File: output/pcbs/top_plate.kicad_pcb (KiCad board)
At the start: 2 copper layers, 162.1 x 157 mm, 0 parts

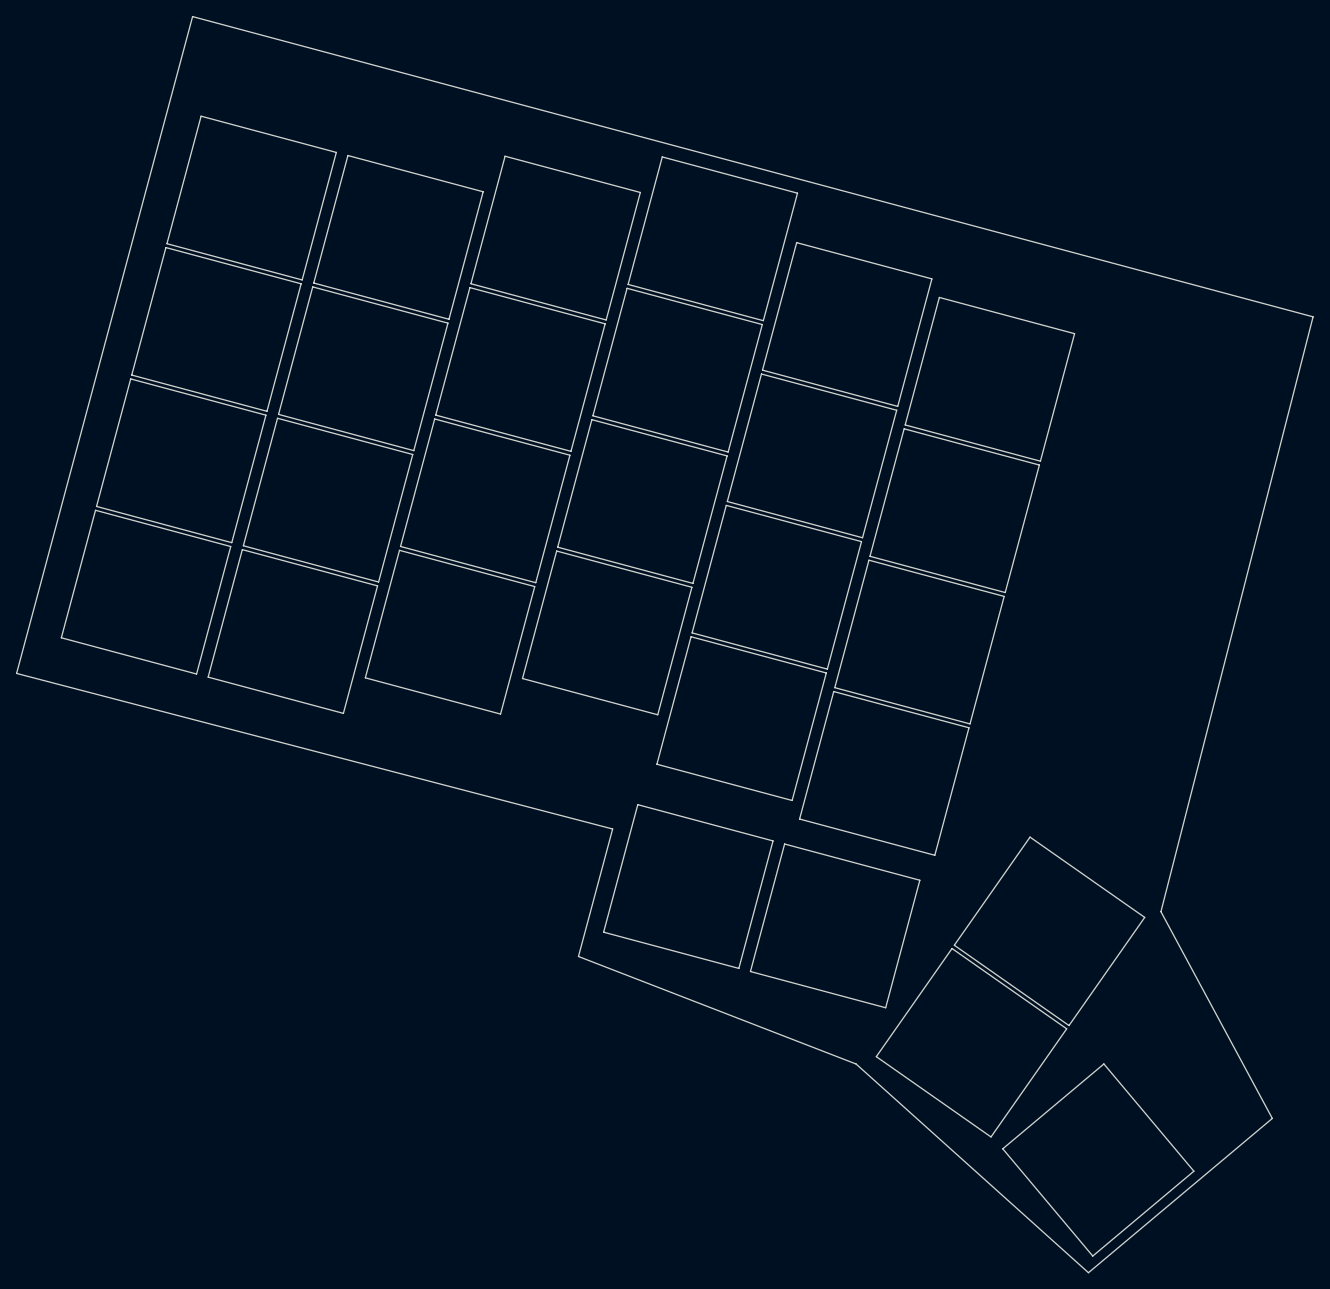
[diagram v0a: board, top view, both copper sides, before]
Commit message: holes
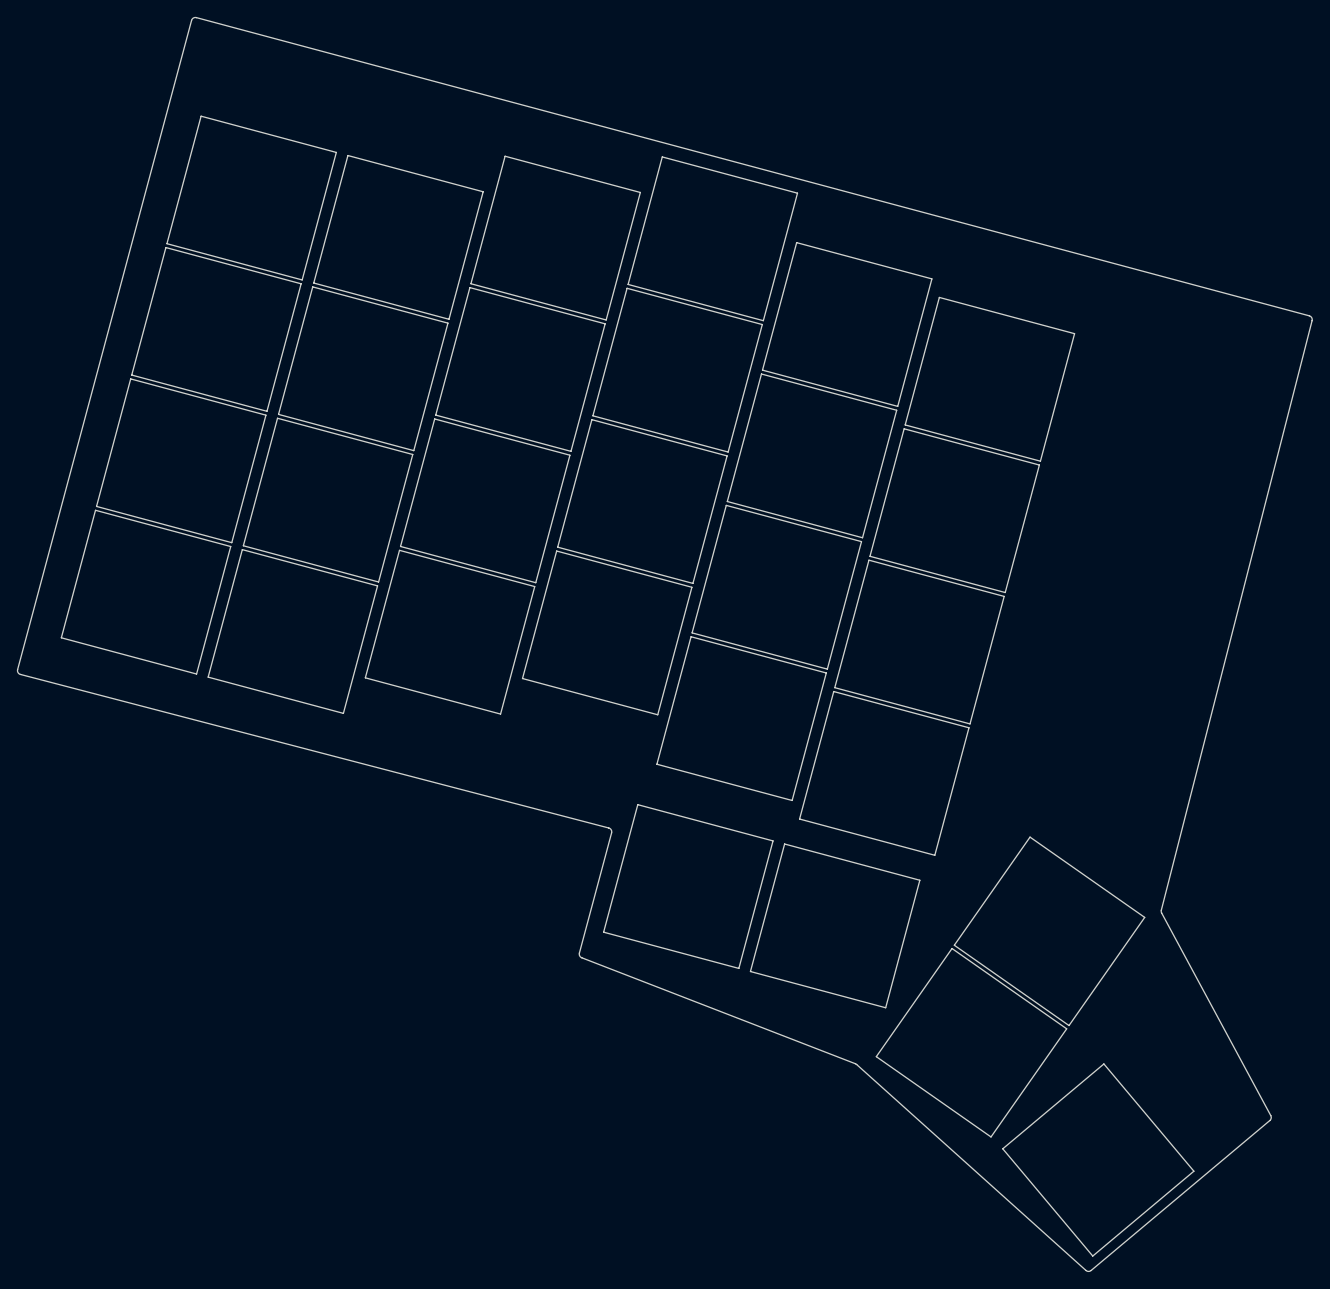
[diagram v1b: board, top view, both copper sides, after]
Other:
- board size 162.1 x 157 mm -> 161.8 x 156.7 mm
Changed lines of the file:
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@@
     (add_net "")
   )
-            (gr_line (start -16.1805024 10.158314) (end 5.819116599999999 -71.94538130000001) (angle 90) (layer Edge.Cuts) (width 0.15))
-(gr_line (start 5.819116599999999 -71.94538130000001) (end 145.87836140000002 -34.4166198) (angle 90) (layer Edge.Cuts) (width 0.15))
-(gr_line (start 145.87836140000002 -34.4166198) (end 126.8621417 39.9409735) (angle 90) (layer Edge.Cuts) (width 0.15))
-(gr_line (start 126.8621417 39.9409735) (end 140.7847307 65.7853827) (angle 90) (layer Edge.Cuts) (width 0.15))
-(gr_line (start 140.7847307 65.7853827) (end 117.80339740000001 85.06901099999999) (angle 90) (layer Edge.Cuts) (width 0.15))
-(gr_line (start 117.80339740000001 85.06901099999999) (end 88.758661 58.982201599999996) (angle 90) (layer Edge.Cuts) (width 0.15))
-(gr_line (start 88.758661 58.982201599999996) (end 54.054681599999995 45.5421936) (angle 90) (layer Edge.Cuts) (width 0.15))
-(gr_line (start 54.054681599999995 45.5421936) (end 58.325195799999996 29.604417499999997) (angle 90) (layer Edge.Cuts) (width 0.15))
-(gr_line (start 58.325195799999996 29.604417499999997) (end -16.1805024 10.158314) (angle 90) (layer Edge.Cuts) (width 0.15))
+            (gr_line (start -16.050249842682216 9.672204841561154) (end 5.6897070767034235 -71.46241838733955) (angle 90) (layer Edge.Cuts) (width 0.15))
+(gr_line (start 6.302079476703429 -71.81597178733956) (end 145.400885349558 -34.54455912199612) (angle 90) (layer Edge.Cuts) (width 0.15))
+(gr_line (start 145.75588576462945 -33.93771318092877) (end 126.91051278171823 39.75183195248809) (angle 90) (layer Edge.Cuts) (width 0.15))
+(gr_line (start 126.95473240803616 40.11284901443227) (end 140.59163301925636 65.42693676176896) (angle 90) (layer Edge.Cuts) (width 0.15))
+(gr_line (start 140.47283653050286 66.04709298264581) (end 118.13593657307975 84.78997750245881) (angle 90) (layer Edge.Cuts) (width 0.15))
+(gr_line (start 117.48043880075463 84.77894262731525) (end 88.82679495778186 59.04339676961162) (angle 90) (layer Edge.Cuts) (width 0.15))
+(gr_line (start 88.67326060229512 58.94912810098919) (end 54.47324822304958 45.70429428296431) (angle 90) (layer Edge.Cuts) (width 0.15))
+(gr_line (start 54.17085493988792 45.10862878948538) (end 58.19494324450718 30.090526658915167) (angle 90) (layer Edge.Cuts) (width 0.15))
+(gr_line (start 57.83825107910054 29.477324167944097) (end -15.69355767727557 10.285407332532225) (angle 90) (layer Edge.Cuts) (width 0.15))
+(gr_arc (start 6.172669976703426 -71.33300888733956) (end 6.302079476703426 -71.81597178733956) (angle -90.00000000000094) (layer Edge.Cuts) (width 0.15))
+(gr_arc (start 145.27147584955802 -34.06159622199612) (end 145.75588574955802 -33.93771322199612) (angle -89.34536259454504) (layer Edge.Cuts) (width 0.15))
+(gr_arc (start 127.39492269678965 39.87571499355545) (end 126.91051279678965 39.75183199355545) (angle -42.65706137359828) (layer Edge.Cuts) (width 0.15))
+(gr_arc (start 140.15144273050288 65.66407078264578) (end 140.4728365305029 66.04709298264578) (angle -78.31169972246471) (layer Edge.Cuts) (width 0.15))
+(gr_arc (start 117.81454277307972 84.40695530245878) (end 117.48043887307972 84.77894260245878) (angle -81.92890097930959) (layer Edge.Cuts) (width 0.15))
+(gr_arc (start 88.49269098545678 59.41538409446811) (end 88.82679488545678 59.04339679446811) (angle -20.75872474796588) (layer Edge.Cuts) (width 0.15))
+(gr_arc (start 54.65381783988792 45.23803828948539) (end 54.170854939887924 45.10862878948539) (angle -83.82982282525415) (layer Edge.Cuts) (width 0.15))
+(gr_arc (start 57.71198034450719 29.961117158915158) (end 58.194943244507186 30.09052665891516) (angle -90.37204223967748) (layer Edge.Cuts) (width 0.15))
+(gr_arc (start -15.567286942682214 9.801614341561148) (end -16.050249842682213 9.672204841561149) (angle -90.37204223967527) (layer Edge.Cuts) (width 0.15))
 (gr_line (start -10.5871081 5.7042214) (end 6.316593900000001 10.2335547) (angle 90) (layer Edge.Cuts) (width 0.15))
 (gr_line (start 6.316593900000001 10.2335547) (end 10.587108100000002 -5.7042214) (angle 90) (layer Edge.Cuts) (width 0.15))
